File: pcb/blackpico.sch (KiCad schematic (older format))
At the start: 3 parts, among them U1 RP2040

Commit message: Hmmmm
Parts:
- added C1, C3: 10uF, Capacitor_SMD:C_0603_1608Metric, symbol Device:C
- added C10, C11, C2, C4, C5, C6, C7: 100nF, Capacitor_SMD:C_0402_1005Metric, symbol Device:C
- added C8, C9: 15pF, Capacitor_SMD:C_0402_1005Metric, symbol Device:C
- added D1: ~, Diode_SMD:D_SOD-123, symbol Device:D_Schottky
- added D2: GRE, LED_SMD:LED_0603_1608Metric, symbol Device:LED
- added D3: BLUE, LED_SMD:LED_0603_1608Metric, symbol Device:LED
- added J3: USB-C, blackpico:USB_C_Receptacle_HRO_TYPE-C-31-M-12, symbol blackpico:USB_C_Receptacle_USB2.0
- added J4: ~, Connector_PinHeader_2.54mm:PinHeader_2x03_P2.54mm_Horizontal, symbol Connector_Generic:Conn_02x03_Odd_Even
- added R1, R4: 10k, Resistor_SMD:R_0402_1005Metric, symbol Device:R
- added R2, R3: 22R, Resistor_SMD:R_0402_1005Metric, symbol Device:R
- added R5, R7: 5.1k, Resistor_SMD:R_0402_1005Metric, symbol Device:R
- added R6, R8: 220, Resistor_SMD:R_0402_1005Metric, symbol Device:R
- added SW1, SW2: TS-1088R-02526, blackpico:TS-1088R-02526, symbol Switch:SW_Push
- added U3: XC6206P332MR, Package_TO_SOT_SMD:SOT-23, symbol Regulator_Linear:XC6206PxxxMR
- added U4: W25Q32JVSS, Package_SO:SOIC-8_5.23x5.23mm_P1.27mm, symbol Memory_Flash:W25Q32JVSS
- added Y1: 12MHz, Crystal:Crystal_SMD_3225-4Pin_3.2x2.5mm, symbol Device:Crystal_GND24
- J1, J2: footprint Connector_PinHeader_2.54mm:PinHeader_2x20_P2.54mm_Vertical -> blackpico:PinSocket_2x20_P2.54mm_Vertical_Stackable
- U1: footprint Package_DFN_QFN:QFN-56-1EP_7x7mm_P0.4mm_EP5.6x5.6mm_ThermalVias -> blackpico:QFN-56-1EP_7x7mm_P0.4mm_EP3.4x3.4mm
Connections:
- net labels added: +1V1, BO0, C13, D+, D-, IO0, IO1, IO10, IO11, IO12, IO13, IO14, IO15, IO16, IO17, IO18, IO19, IO2, IO20, IO21, IO22, IO26, IO27, IO28, IO3, IO4, IO5, IO6, IO7, IO8, IO9, QCK, QD0, QD1, QD2, QD3, QSS, RST, RUN, SWCLK, SWDIO, SWO, VDC, XI, XO
- net labels removed: VPP
- wire segments 0 -> 251
- no-connect marks 0 -> 2
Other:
- note added: "Decoupling"
- note added: "Green: 3.3V\nBlue: PC13"
- note added: "Internal pull-up"
- note added: "LEDs"
- note added: "Power Regulation"
- note added: "Programming Header"
- note added: "Reset & Boot Mode"
- note added: "USB C Connection"
- moved on the sheet: J1, J2, U1

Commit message: Hmmmmm
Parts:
- added C12: 2.2uF, Capacitor_SMD:C_0402_1005Metric, symbol Device:C
- added C13: 100nF, Capacitor_SMD:C_0402_1005Metric, symbol Device:C
- added D4, D5, D6, D7: WS2812B, blackpico:WS2812B-2020, symbol blackpico:WS2812B-2020
- U4: value W25Q32JVSS -> W25Q128JVSIQ; LCSC (none) -> C97521
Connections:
- net labels added: ADC_VREF, RGB
- wire segments 251 -> 279
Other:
- moved on the sheet: C10, C11, C4, C5, C6, C7, C8, C9, D1, D2, D3, J2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

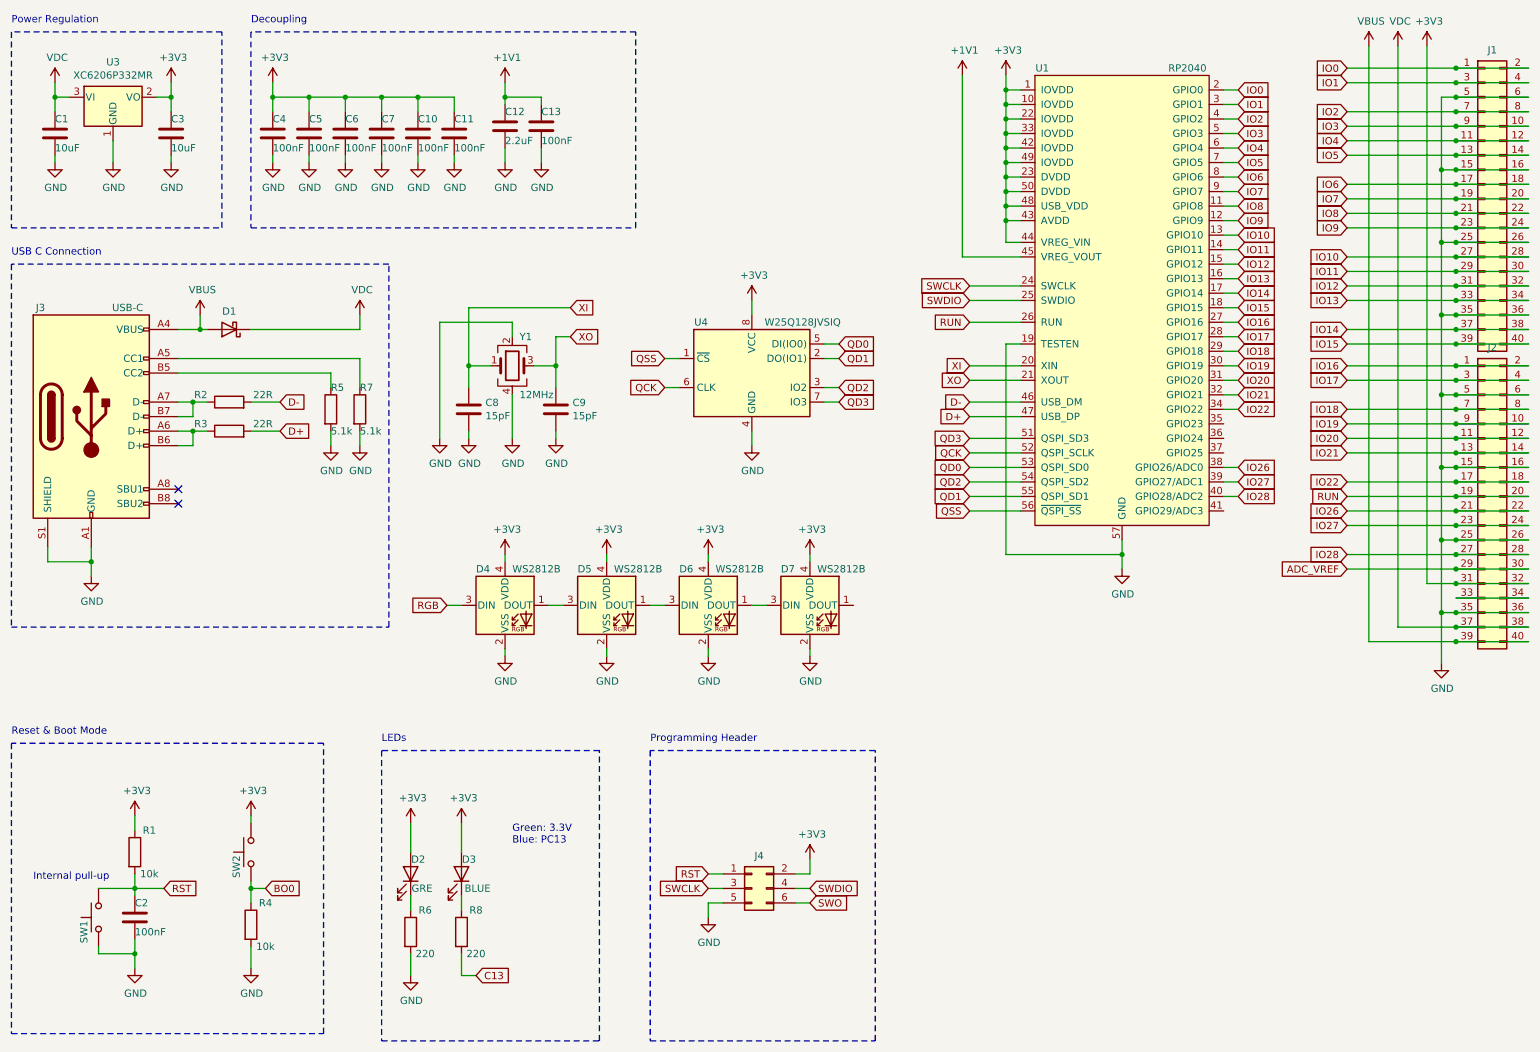
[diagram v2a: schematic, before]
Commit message: Hmmmm
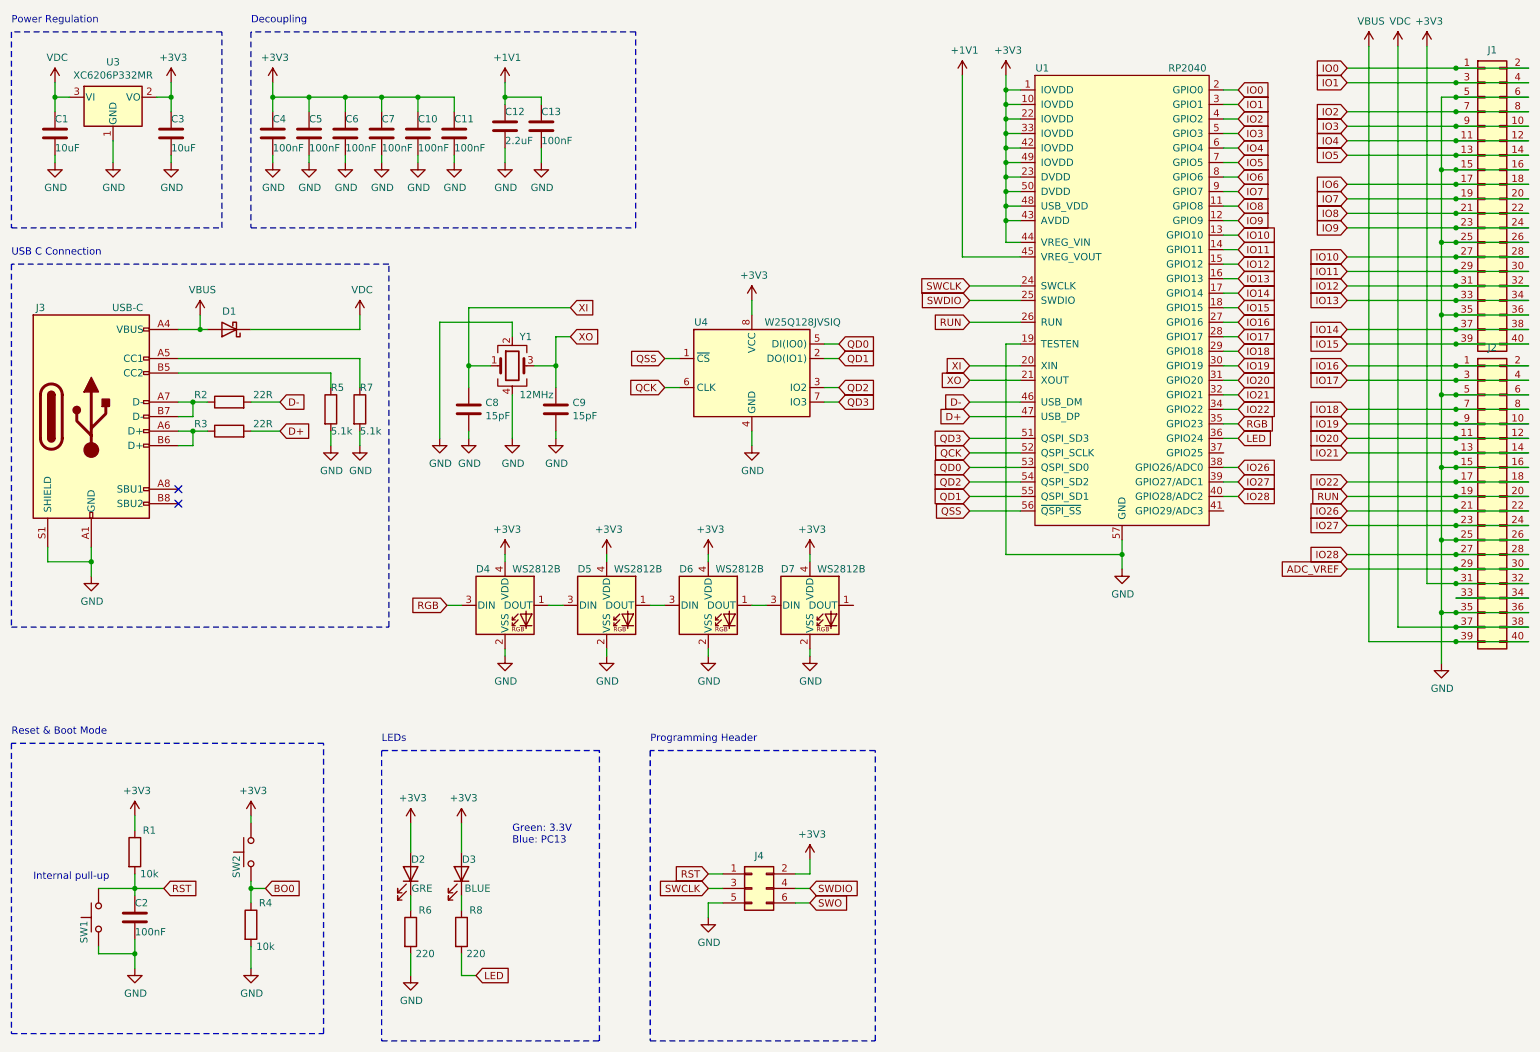
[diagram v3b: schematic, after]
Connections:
- net C13 is gone; now on net LED: R8.2
- net RGB: now also U1.35 (GPIO23)
- net LED: now reaches U1.36 (GPIO24)
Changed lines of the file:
@@
 	3400 7200 3400 7050
 Text GLabel 3850 7200 2    50   Input ~ 0
-C13
+LED
 Wire Wire Line
 	3750 6150 3750 6350
@@
 	10600 4500 10400 4500
 Connection ~ 10600 4500
+Text GLabel 9100 3400 2    50   Input ~ 0
+RGB
+Text GLabel 9100 3500 2    50   Input ~ 0
+LED
+Wire Wire Line
+	9100 3400 9000 3400
+Wire Wire Line
+	9000 3500 9100 3500
 $EndSCHEMATC
